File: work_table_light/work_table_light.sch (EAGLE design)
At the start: 8 parts, among them IC1 TINY24/44/84-PU

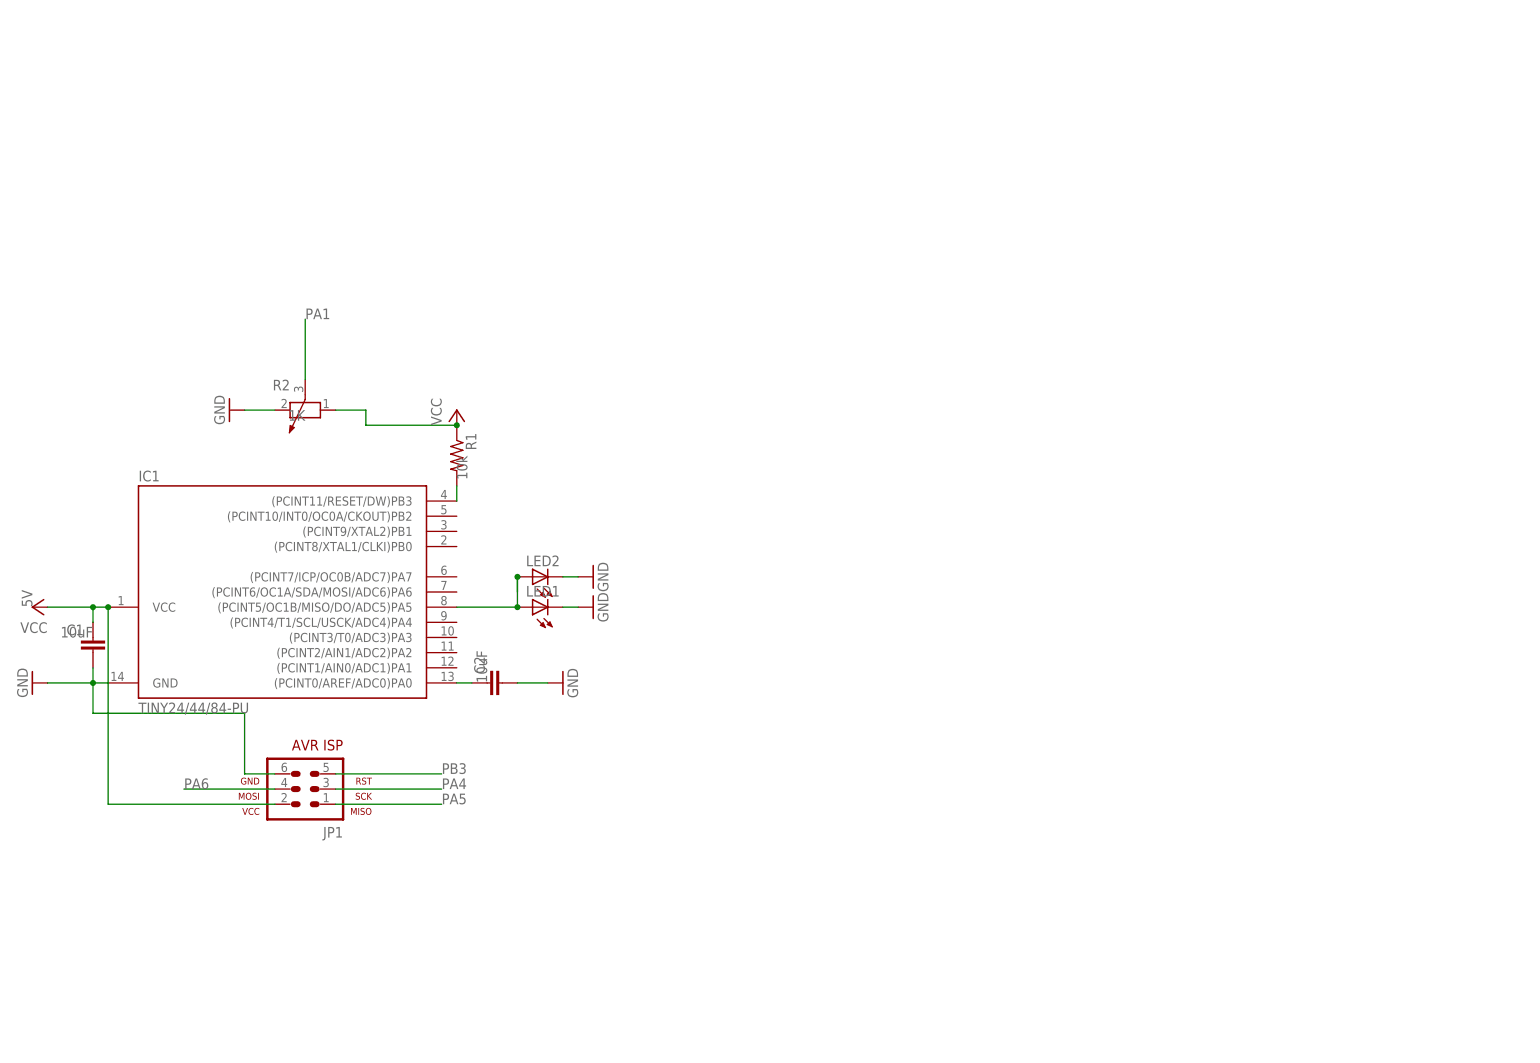
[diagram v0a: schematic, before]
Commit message: schematic updated
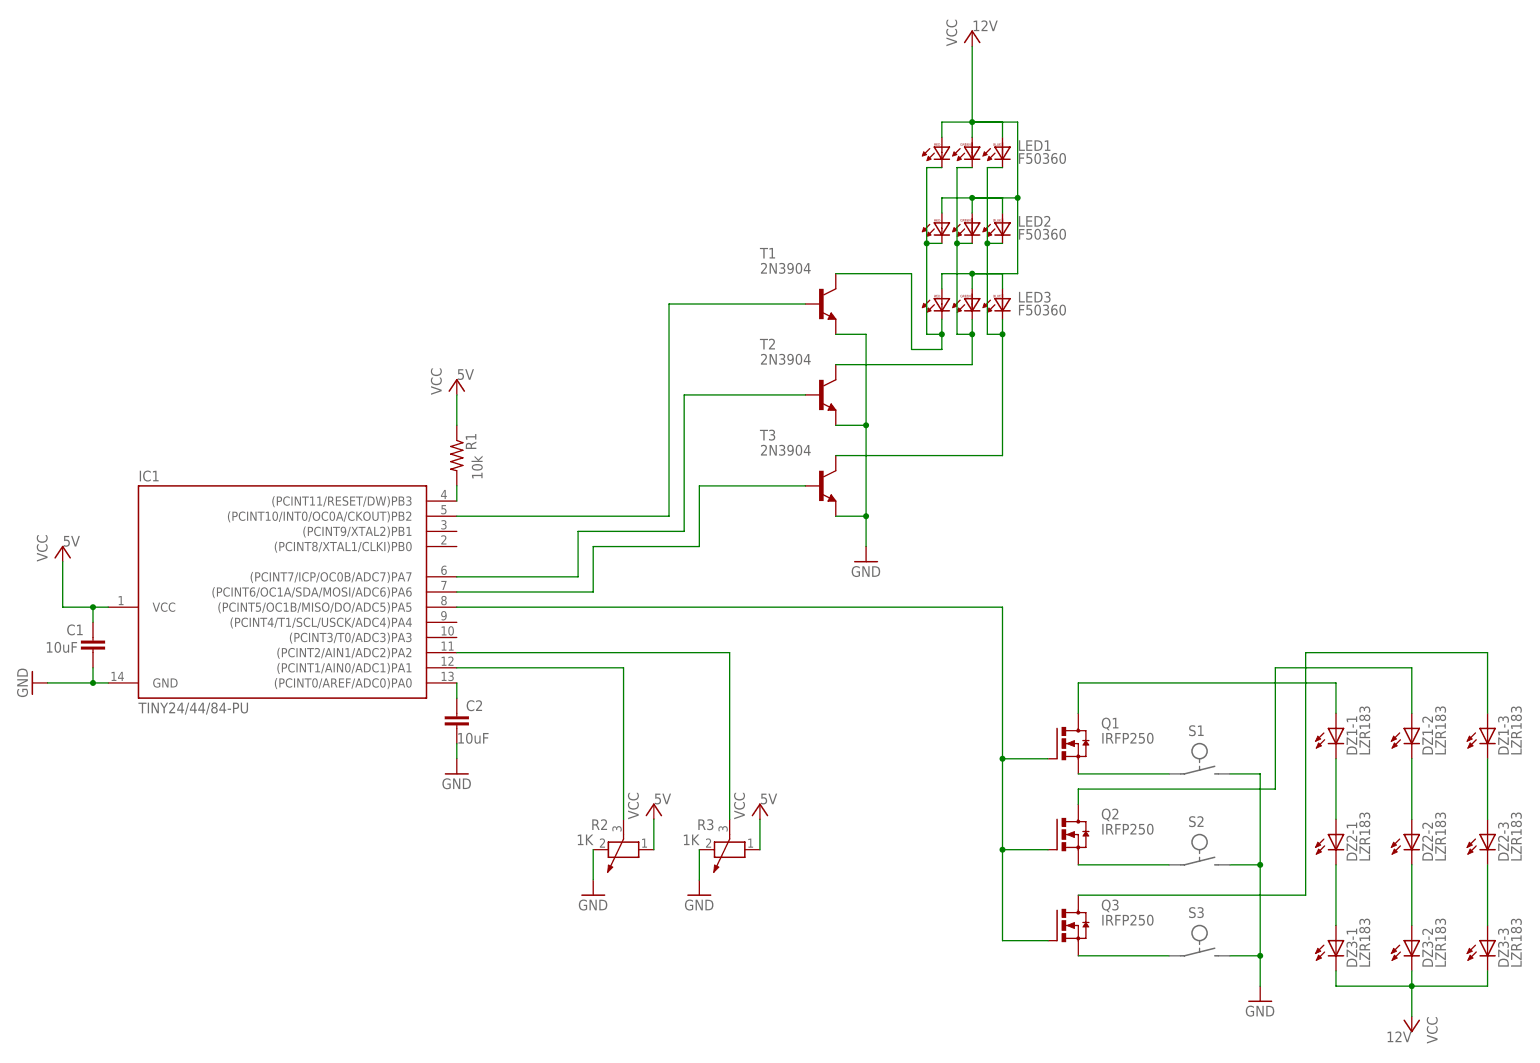
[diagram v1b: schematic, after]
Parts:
- removed JP1: AVR-ISP-6VERT, avr-7:AVR-ISP-6VERT
- added DZ1, DZ2, DZ3: LZR183, led:LZR183
- added LED3: F50360, led:F50360
- added Q1, Q2, Q3: IRFP250, transistor-power:IRFP250
- added R3: (no value), rcl:POTENTIOMETER_PT-10S
- added T1, T2, T3: 2N3904, transistor:2N3904
- LED1, LED2: value (none) -> F50360; device eagle-ltspice:LED_ELD260 -> led:F50360
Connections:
- removed net PA1: R2.3
- removed net PA4: JP1.3
- removed net PA5: JP1.1
- removed net PA6: JP1.4
- removed net PB3: JP1.5
- new net N$1: LED1.RC, LED2.RC, LED3.RC, T1.C
- new net N$10: Q3.S
- new net N$11: DZ1-1.A, Q1.D
- new net N$12: DZ1-1.C, DZ2-1.A
- new net N$13: DZ2-1.C, DZ3-1.A
- new net N$14: DZ1-2.A, Q2.D
- new net N$15: DZ1-2.C, DZ2-2.A
- new net N$16: DZ2-2.C, DZ3-2.A
- new net N$17: DZ1-3.A, Q3.D
- new net N$18: DZ1-3.C, DZ2-3.A
- new net N$19: DZ2-3.C, DZ3-3.A
- new net N$20: IC1.(PCINT10/INT0/OC0A/CKOUT)PB2, T1.B
- new net N$21: LED1.GC, LED2.GC, LED3.GC, T2.C
- new net N$22: LED1.BC, LED2.BC, LED3.BC, T3.C
- new net N$23: IC1.(PCINT1/AIN0/ADC1)PA1, R2.3
- new net N$4: IC1.(PCINT6/OC1A/SDA/MOSI/ADC6)PA6, T3.B
- new net N$5: IC1.(PCINT7/ICP/OC0B/ADC7)PA7, T2.B
- new net N$6: IC1.(PCINT2/AIN1/ADC2)PA2, R3.3
- new net N$7: Q1.S
- new net N$8: Q2.S
- net GND: now also R3.2, T1.E, T2.E, T3.E; no longer JP1.6, LED1.C, LED2.C
- net N$2: now also Q1.G, Q2.G, Q3.G; no longer LED1.A, LED2.A
- net VCC: now also DZ3-1.C, DZ3-2.C, DZ3-3.C, LED1.BA, LED1.GA, LED1.RA, LED2.BA, LED2.GA, LED2.RA, LED3.BA, LED3.GA, LED3.RA, R3.1; no longer JP1.2
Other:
- moved on the sheet: C2, R2
